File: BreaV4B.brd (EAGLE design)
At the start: 30.8 x 19 mm, 32 parts, among them J1 XF2L-0535-1, J2 XF2L-0535-1, Q3 ABM-16MHZ, SW1 ESE31L11T, SW2 EVQ11U09K, SW3 LS12T2-T, U1 TPS62200, X1 22-23-2021

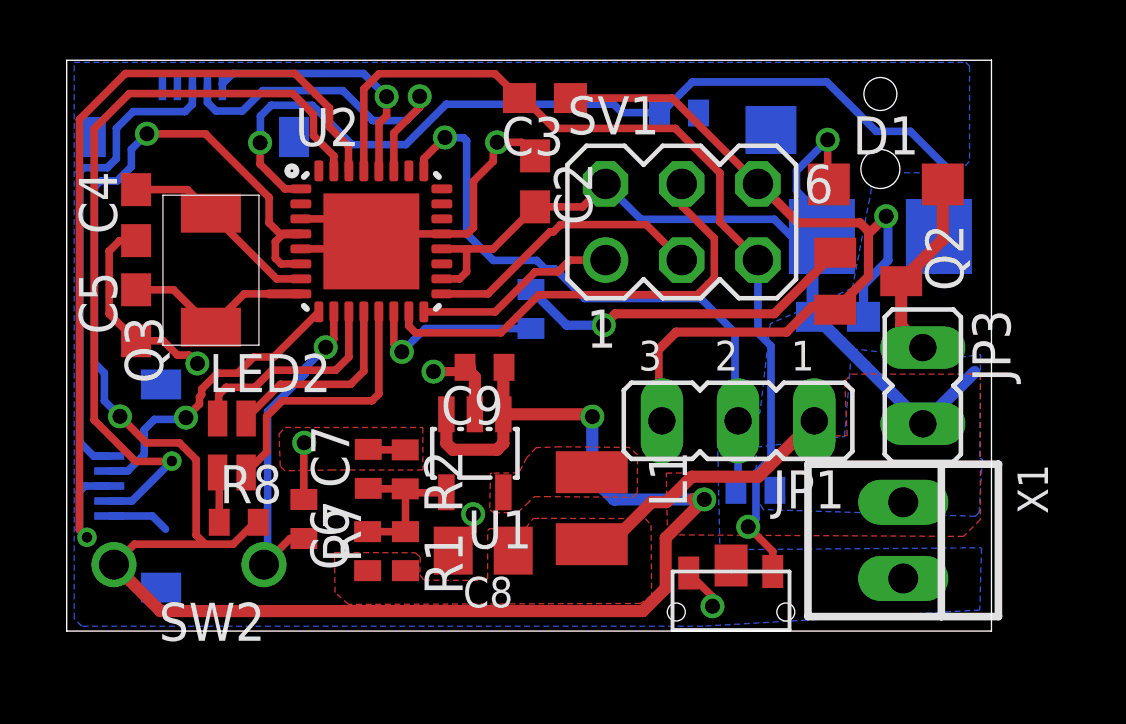
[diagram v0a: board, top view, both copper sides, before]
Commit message: TrussKey Schematics
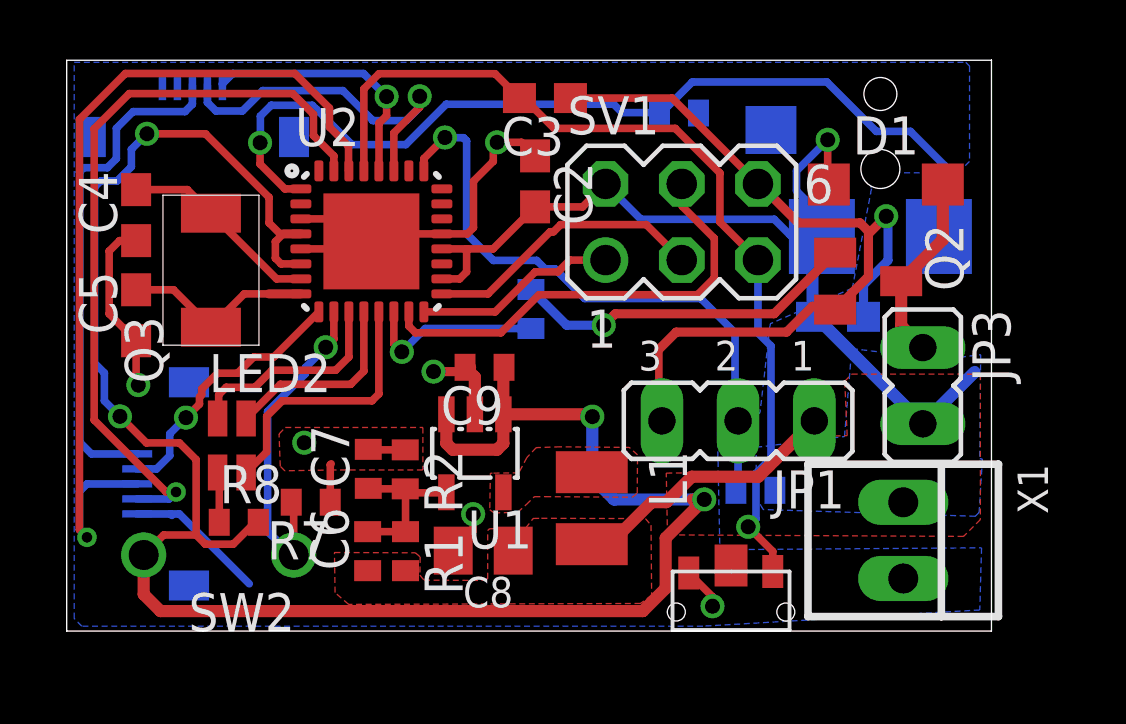
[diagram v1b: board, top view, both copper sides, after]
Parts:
- R8: value 10K -> 1K
- moved SW2 1.04 mm to (5.07, 2.50)
- moved J1 0.93 mm to (4.26, 4.87)
- moved R7 0.61 mm to (8.14, 4.26), turned to 180 degrees
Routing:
- net VCC: track 101.8 -> 100.4 mm
- net GND: track 60.4 -> 61.7 mm
- net REST: track 9.92 -> 8.90 mm
- net RX: track 28.5 -> 29.5 mm
- net VBATSIM: track 16.1 -> 17.0 mm
- net TX: track 25.9 -> 25.1 mm
